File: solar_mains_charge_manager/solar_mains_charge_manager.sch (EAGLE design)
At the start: 32 parts, among them T1 TIP122, X10 22-23-2041, X2 22-23-2021, X3 22-23-2031, X5 22-23-2031, X6 22-23-2041, X7 53047-15, X8 53047-15

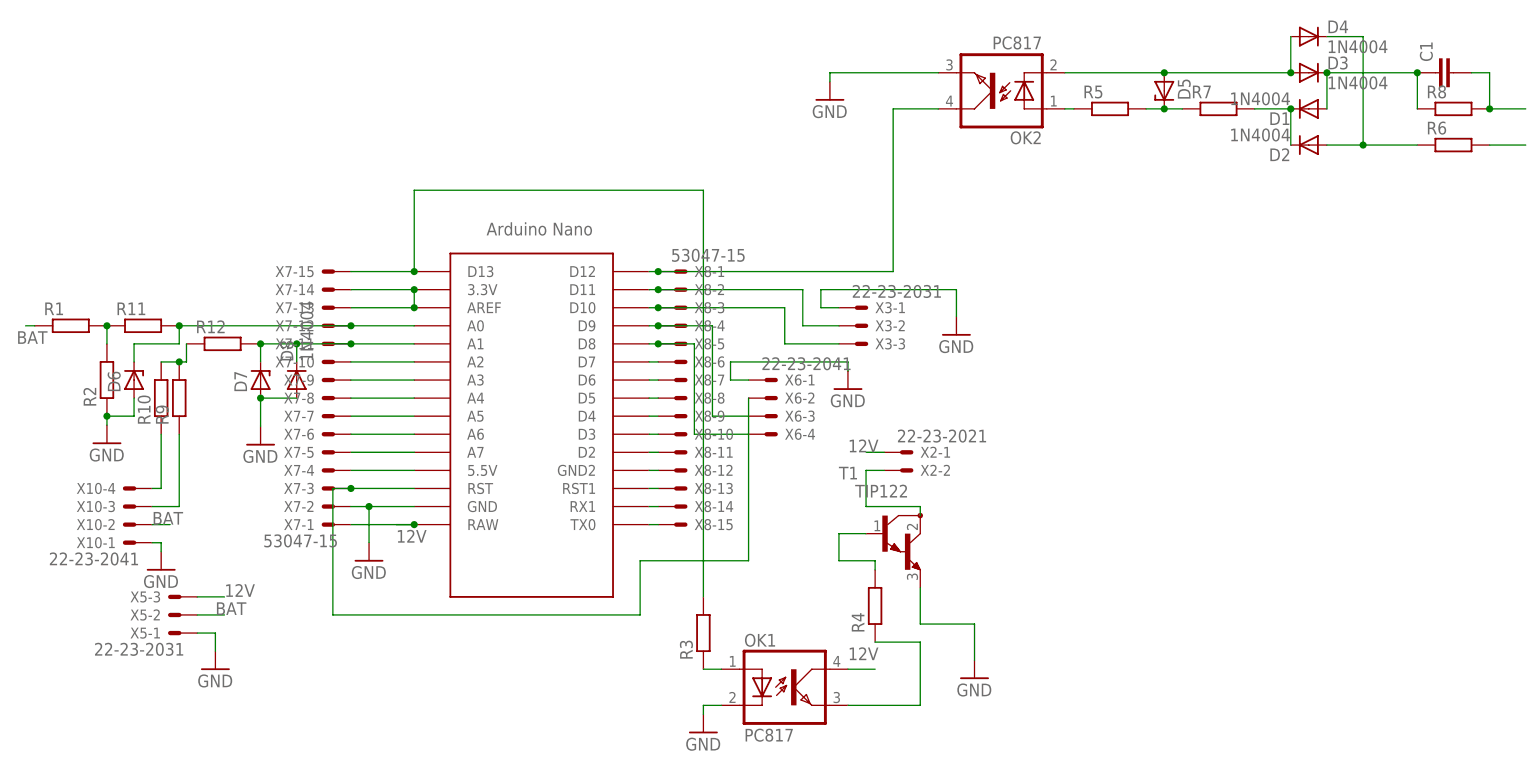
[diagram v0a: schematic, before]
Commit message: A lot of stuff
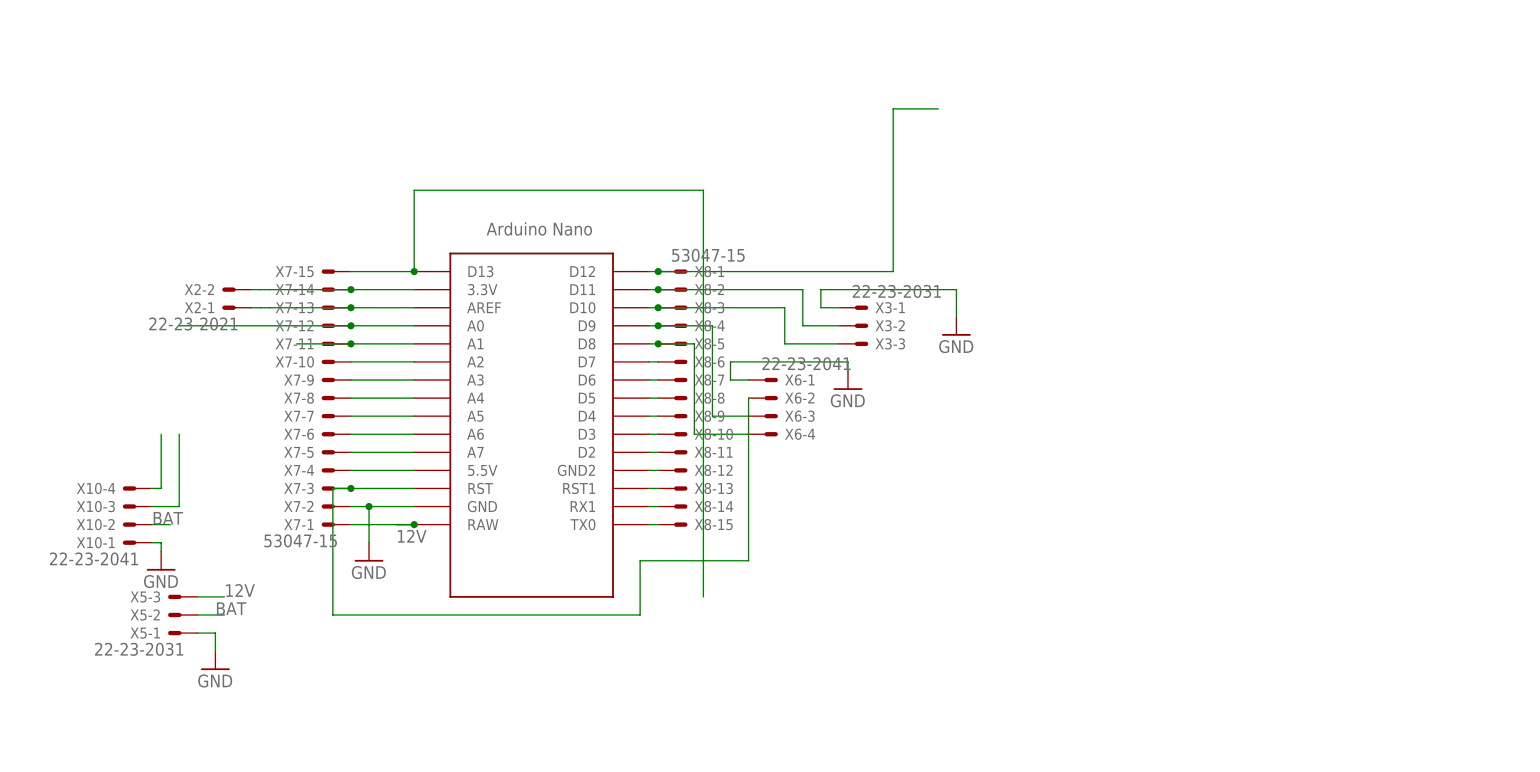
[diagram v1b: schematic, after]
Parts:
- removed C1: (no value), capacitor-wima:C5/2.5
- removed D1, D2, D3, D4, D8: 1N4004, diode:1N4004
- removed D5, D6, D7: (no value), diode:ZENER-DIODEDO34-7
- removed OK1, OK2: PC817, optocoupler:PC817
- removed R1, R10, R11, R12, R2, R3, R4, R5, R9: (no value), resistor:R-EU_0204/5
- removed R6, R7, R8: (no value), resistor:R-EU_0204/7
- removed T1: TIP122, transistor:TIP122
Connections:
- removed net N$1: U$1.3.3V, U$1.AREF, X7-13.S, X7-14.S
- removed net N$10: D3.A, D4.A, D5.A, OK2.C
- removed net N$11: D1.C, D2.C, R7.2
- removed net N$13: C1.1, D1.A, D3.C, R8.1
- removed net N$14: C1.2, R8.2
- removed net N$15: D2.A, D4.C, R6.1
- removed net N$16: R6.2
- removed net N$3: R10.2, R12.1, R9.2
- removed net N$4: OK1.A, R3.1
- removed net N$43: R1.2, R11.1, R2.2
- removed net N$6: OK1.EMIT, R4.1
- removed net N$7: R4.2, T1.B
- removed net N$8: OK2.A, R5.1
- removed net N$9: D5.C, R5.2, R7.1
- new net 12V1: U$1.AREF, X2-1.S, X7-13.S
- net 12V: no longer OK1.COL, X2-1.S
- net BAT: no longer R1.1
- net GND: no longer D6.A, D7.A, D8.A, OK1.C, OK2.EMIT, R2.1, T1.E
- net N$12: no longer OK2.COL
- net N$2: no longer R3.2
- net N$39: no longer D7.C, D8.C, R12.2
- net N$40: no longer D6.C, R11.2
- net N$41: no longer R10.1
- net N$42: no longer R9.1
- net N$5: now also U$1.3.3V, X7-14.S; no longer T1.C
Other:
- moved on the sheet: X2-1, X2-2

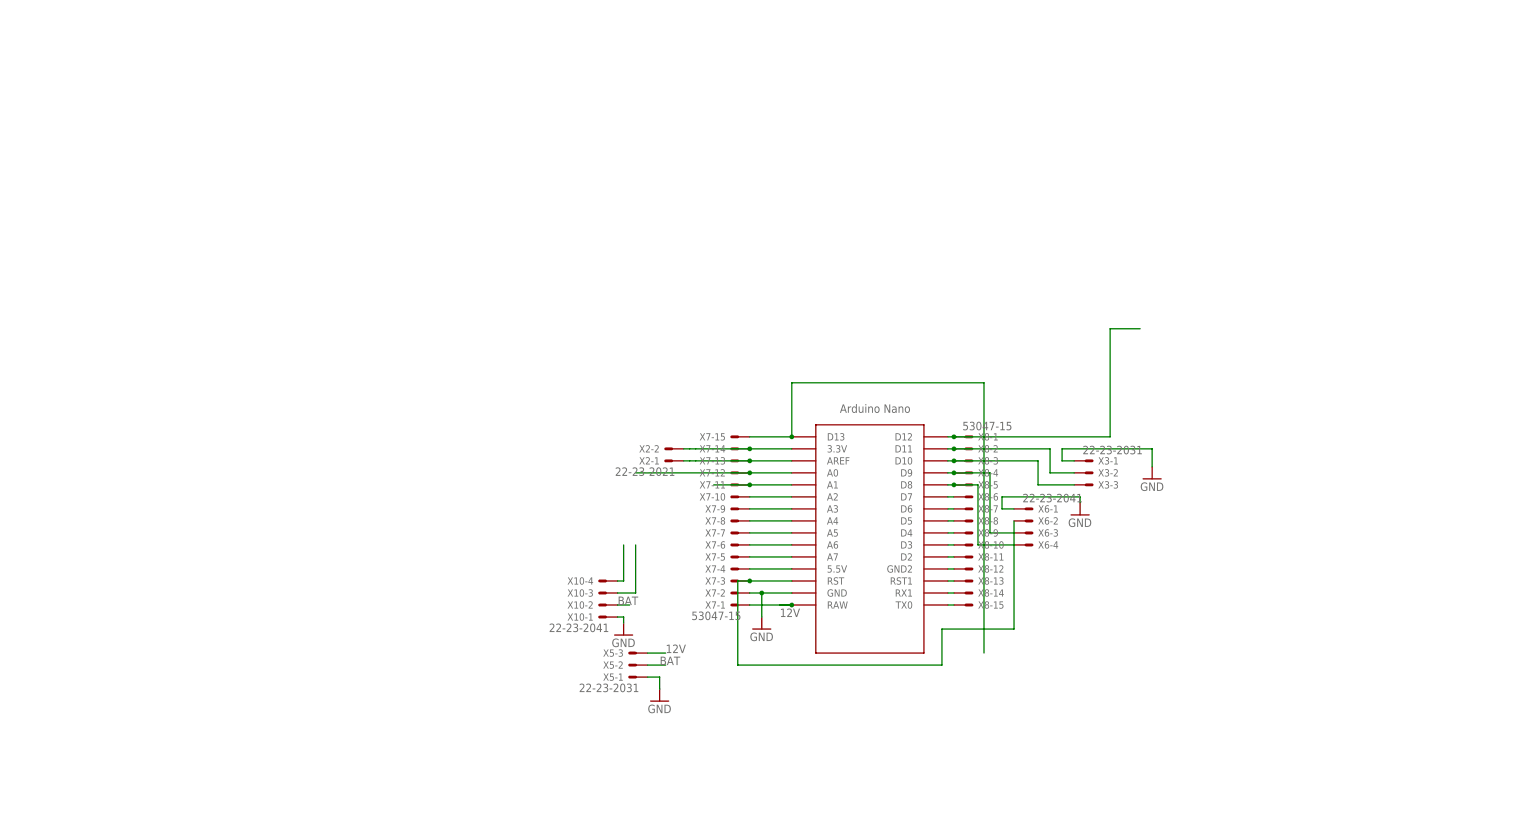
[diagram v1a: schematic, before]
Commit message: Stuff
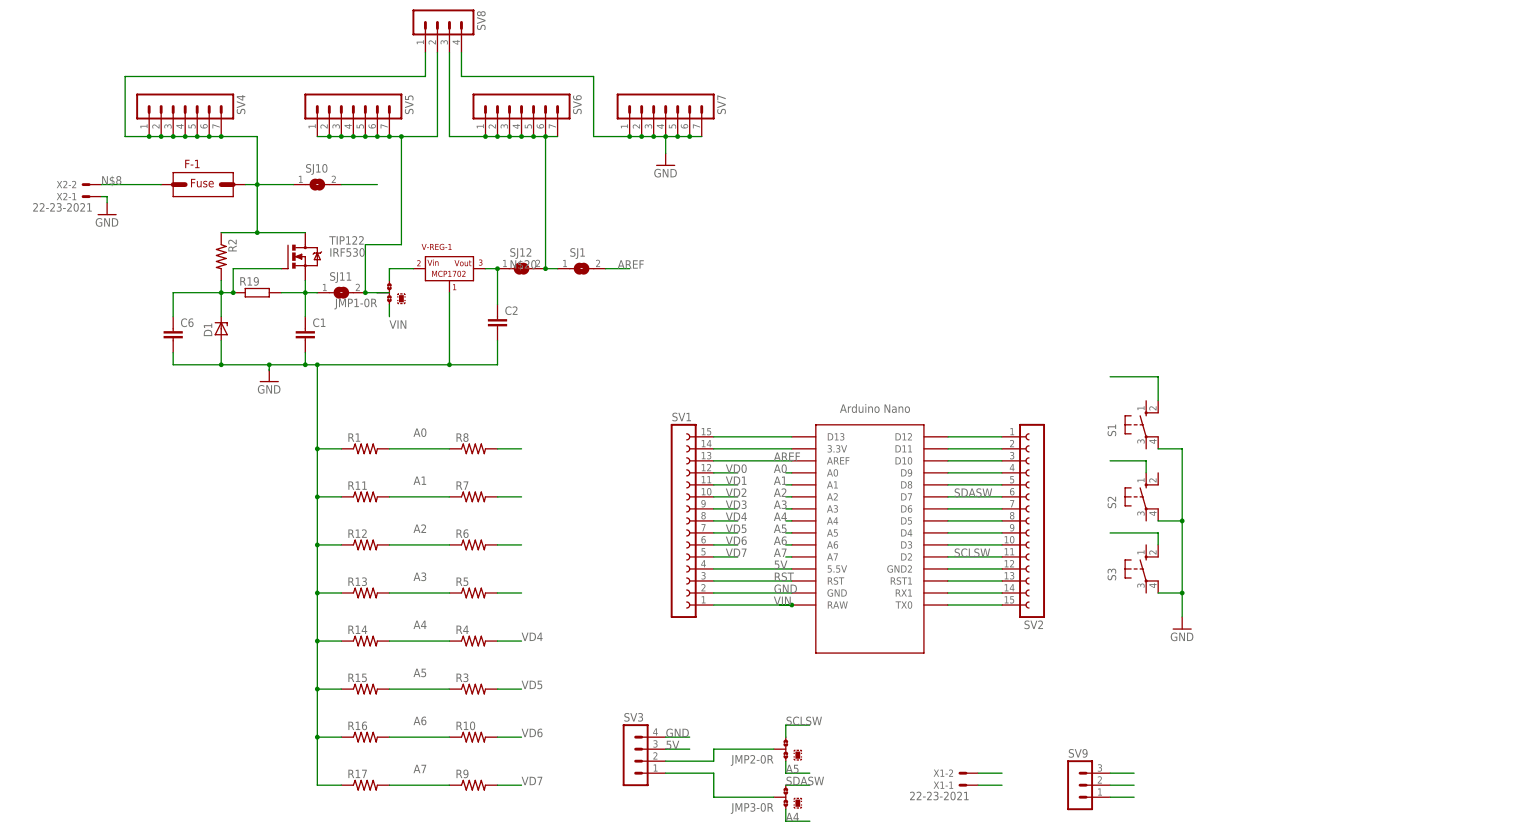
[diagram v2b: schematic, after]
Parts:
- removed X10, X6: 22-23-2041, con-molex:22-23-2041
- removed X3, X5: 22-23-2031, con-molex:22-23-2031
- removed X7, X8: 53047-15, con-molex:53047-15
- added C1, C2, C6: (no value), capacitor-wima:C2,5-3
- added D1: (no value), diode:ZENER-DIODEDO34-7
- added F-1: (no value), qfm-trx1-24g:FUSE
- added JMP1, JMP2, JMP3: 0R-JUMPA, jump-0r-smd:0R-JUMPA
- added R1, R11, R12, R13, R14, R15, R16, R17: (no value), rcl:R-US_0204/5
- added R10, R2, R3, R4, R5, R6, R7, R8, R9: (no value), resistor:R-US_0204/2V
- added R19: (no value), resistor:R-EU_0204/5
- added S1, S2, S3: (no value), switch-omron:10-XX
- added SJ1, SJ10, SJ11, SJ12: (no value), jumper:SJ
- added SV1, SV2: (no value), con-lsta:FE15-1
- added SV3, SV8: (no value), con-lstb:MA04-1
- added SV4, SV5, SV6, SV7: (no value), con-lstb:MA07-1
- added SV9: (no value), con-lstb:MA03-1
- added TIP122: IRF530, transistor-power:IRF530
- added V-REG-1: (no value), qfm-trx1-24g:MCP1702
- added X1: 22-23-2021, con-molex:22-23-2021
- U$1: device Arduino-clone:NANO -> nano_without_those_headers:NANO
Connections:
- removed net 12V: U$1.RAW, X5-3.S, X7-1.S
- removed net 12V1: U$1.AREF, X2-1.S, X7-13.S
- removed net N$17: U$1.D11, X3-2.S, X8-2.S
- removed net N$19: U$1.D9, X6-3.S, X8-4.S
- removed net N$22: U$1.D7, X8-6.S
- removed net N$23: U$1.D6, X8-7.S
- removed net N$27: U$1.D2, X8-11.S
- removed net N$28: U$1.GND2, X8-12.S
- removed net N$32: U$1.5.5V, X7-4.S
- removed net N$33: U$1.A7, X7-5.S
- removed net N$34: U$1.A6, X7-6.S
- removed net N$35: U$1.A5, X7-7.S
- removed net N$36: U$1.A4, X7-8.S
- removed net N$37: U$1.A3, X7-9.S
- removed net N$38: U$1.A2, X7-10.S
- removed net N$39: U$1.A1, X7-11.S
- removed net N$40: U$1.A0, X7-12.S
- removed net N$41: X10-4.S
- removed net N$42: X10-3.S
- new net 5V: SJ1.1, SJ12.2, SV1.4, SV3.3, SV6.1, SV6.2, SV6.3, SV6.4, SV6.5, SV6.6, SV6.7, SV8.3, SV9.3, U$1.5.5V
- new net A0: R1.2, R8.1, U$1.A0
- new net A1: R11.2, R7.1, U$1.A1
- new net A2: R12.2, R6.1, U$1.A2
- new net A3: R13.2, R5.1, U$1.A3
- new net A4: JMP3-0R.1, R14.2, R4.1, U$1.A4
- new net A5: JMP2-0R.1, R15.2, R3.1, U$1.A5
- new net A6: R10.1, R16.2, U$1.A6
- new net A7: R17.2, R9.1, SV9.1, U$1.A7
- new net AREF: SJ1.2, SV1.13, U$1.AREF
- new net D8: S2.S, SV2.5, U$1.D8
- new net D9: S1.S1, SV2.4, U$1.D9
- new net N$1: C1.1, R19.2, SJ11.1, TIP122.S
- new net N$13: JMP3-0R.2, SV3.1
- new net N$3: C6.1, D1.C, R19.1, R2.2, TIP122.G
- new net N$4: SV2.1, U$1.D12
- new net N$6: JMP1-0R.3, V-REG-1.P$1
- new net N$7: SV2.2, U$1.D11
- new net N$8: F-1.P$1, X2-2.S
- new net RELAY: SV2.7, U$1.D6, X1-2.S
- new net RST: S3.S1, SV1.3, U$1.RST
- new net SCLSW: JMP2-0R.3, SV2.11, U$1.D2
- new net SDASW: JMP3-0R.3, SV2.6, U$1.D7
- new net VD0: R8.2, SJ10.2, SV1.12
- new net VD1: R7.2, SV1.11
- new net VD2: R6.2, SV1.10
- new net VD3: R5.2, SV1.9
- new net VD4: R4.2, SV1.8
- new net VD5: R3.2, SV1.7
- new net VD6: R10.2, SV1.6
- new net VD7: R9.2, SV1.5
- new net VIN: JMP1-0R.1, SV1.1, U$1.RAW
- net BAT: now also F-1.P$2, R2.1, SJ10.1, SV4.1, SV4.2, SV4.3, SV4.4, SV4.5, SV4.6, SV4.7, SV8.1, TIP122.D; no longer X10-2.S, X5-2.S
- net GND: now also C1.2, C2.2, C6.2, D1.A, R1.1, R11.1, R12.1, R13.1, R14.1, R15.1, R16.1, R17.1, S1.P1, S2.P1, S3.P1, SV1.2, SV2.12, SV3.4, SV7.1, SV7.2, SV7.3, SV7.4, SV7.5, SV7.6, SV7.7, SV8.4, SV9.2, U$1.GND2, V-REG-1.P$2, X1-1.S, X2-1.S; no longer X10-1.S, X3-1.S, X5-1.S, X6-1.S, X7-2.S
- net N$12: now also JMP2-0R.2, SV3.2; no longer U$1.D12, X8-1.S
- net N$18: now also SV2.3; no longer X3-3.S, X8-3.S
- net N$2: now also SV1.15; no longer X7-15.S
- net N$20: now also C2.1, SJ12.1, V-REG-1.P$3; no longer U$1.D8, X6-4.S, X8-5.S
- net N$21: now also JMP1-0R.2, SJ11.2, SV5.1, SV5.2, SV5.3, SV5.4, SV5.5, SV5.6, SV5.7, SV8.2; no longer U$1.RST, X6-2.S, X7-3.S
- net N$24: now also SV2.8; no longer X8-8.S
- net N$25: now also SV2.9; no longer X8-9.S
- net N$26: now also SV2.10; no longer X8-10.S
- net N$29: now also SV2.13; no longer X8-13.S
- net N$30: now also SV2.14; no longer X8-14.S
- net N$31: now also SV2.15; no longer X8-15.S
- net N$5: now also SV1.14; no longer X2-2.S, X7-14.S
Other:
- moved on the sheet: X2-1, X2-2
